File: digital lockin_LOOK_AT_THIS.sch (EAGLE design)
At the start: 24 parts, among them IC1 OPA2650E, IC2 LM358D, T2 NPN, U2 RASPBERRY_PICOSMD-TH, U5 TL431AIDBZR

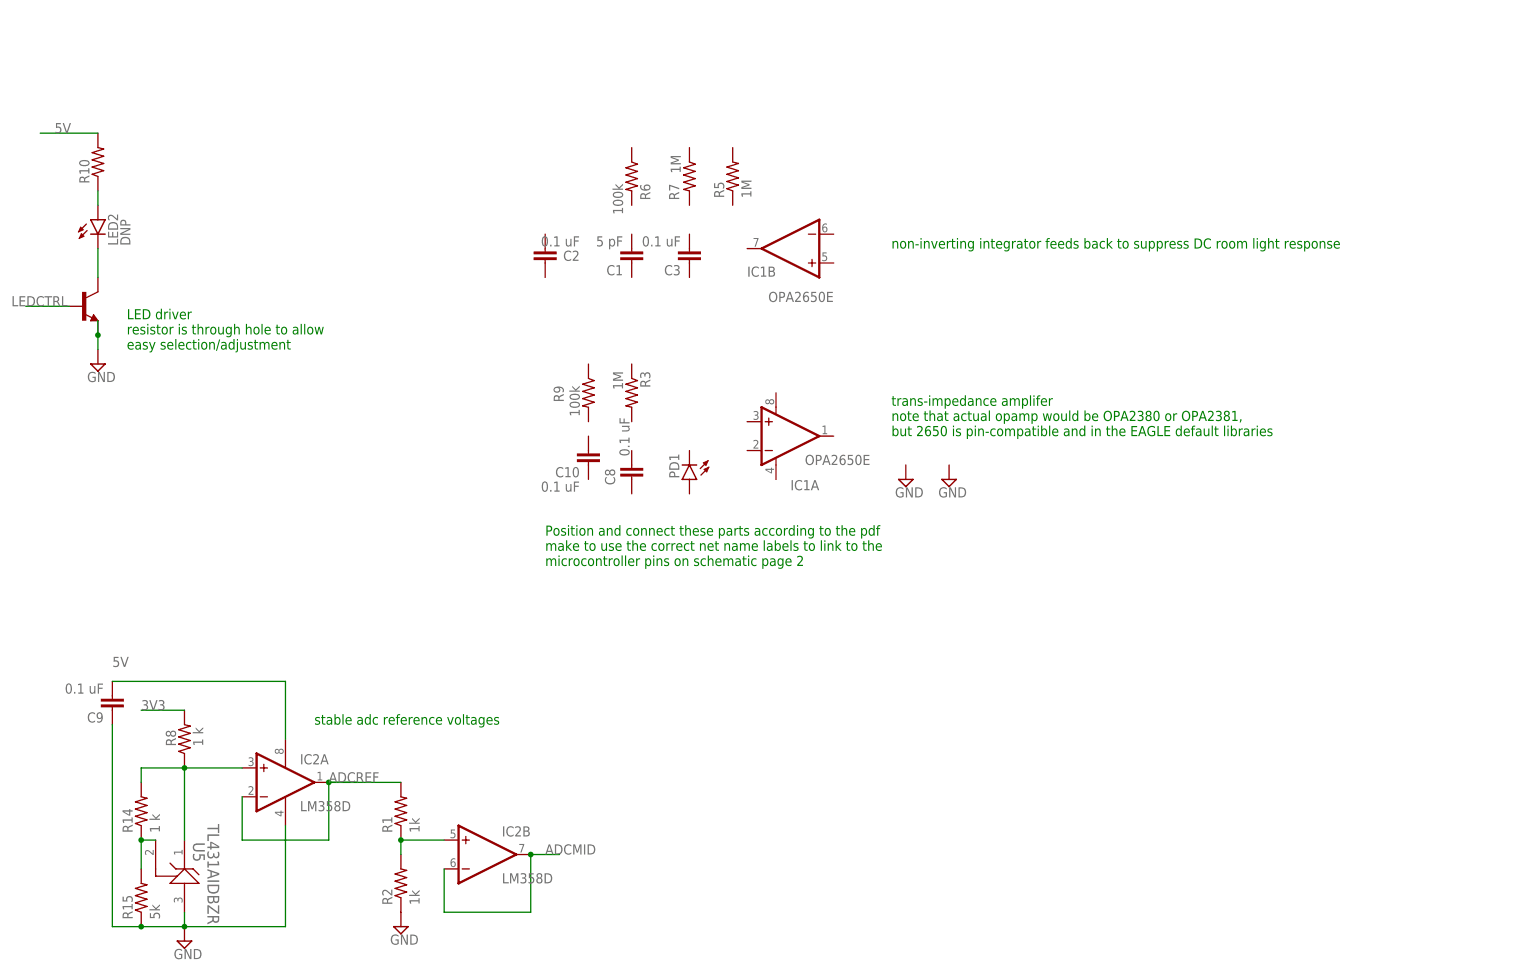
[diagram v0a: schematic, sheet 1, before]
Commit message: UPLOAD
look at this when i upload
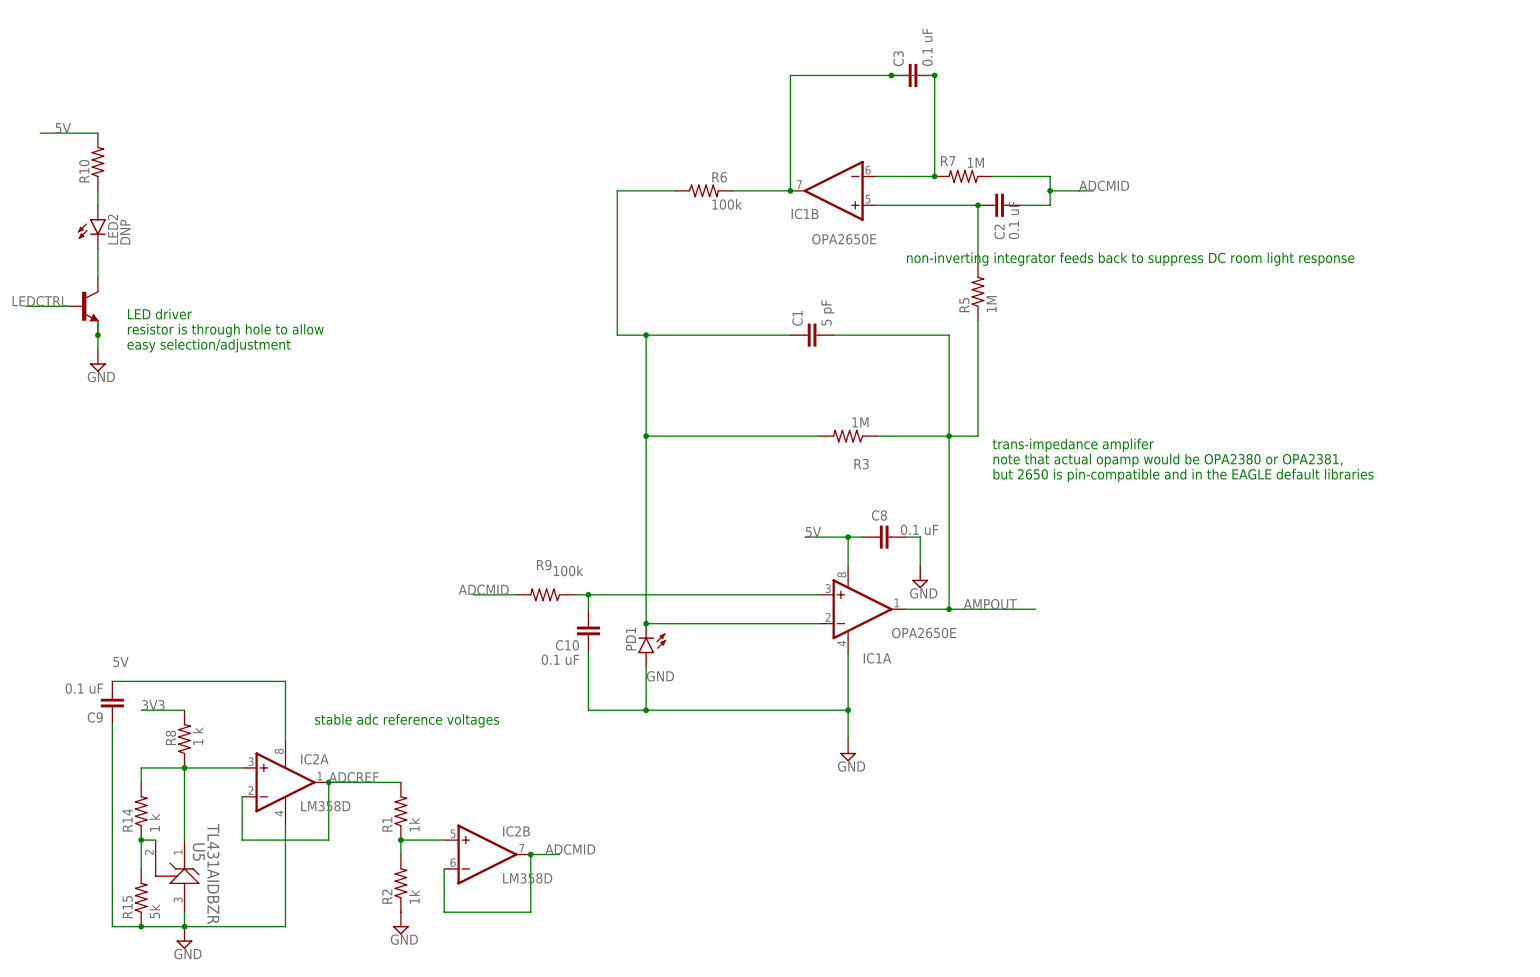
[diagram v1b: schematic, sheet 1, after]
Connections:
- new net N$1: C3.1, C3.2, IC1B.-IN, IC1B.OUT, R6.2, R7.2
- new net N$2: C2.1, IC1B.+IN, R5.2
- new net N$5: C1.1, IC1A.-IN, PD1.C, R3.2, R6.1
- new net N$7: C10.2, IC1A.+IN, R9.1
- net 5V: now also C8.1, IC1A.V+
- net ADCMID: now also C2.2, R7.1, R9.2
- net AMPOUT: now also C1.2, IC1A.OUT, R3.1, R5.1
- net GND: now also C10.1, C8.2, IC1A.V-, PD1.A
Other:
- note removed: "Position and connect these parts according to the pdf make to use the correct net name labels to link to the microcontroller pins on schematic page 2"
- moved on the sheet: C1, C10, C2, C3, C8, IC1A, IC1B, PD1, R3, R5, R6, R7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
